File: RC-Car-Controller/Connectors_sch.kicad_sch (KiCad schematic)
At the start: 6 parts, among them J1 MCU_IF, J3 MOTOR_IF, J4 BATT_1, J5 MISC_IF, J6 ANT_IF, J7 BATT2

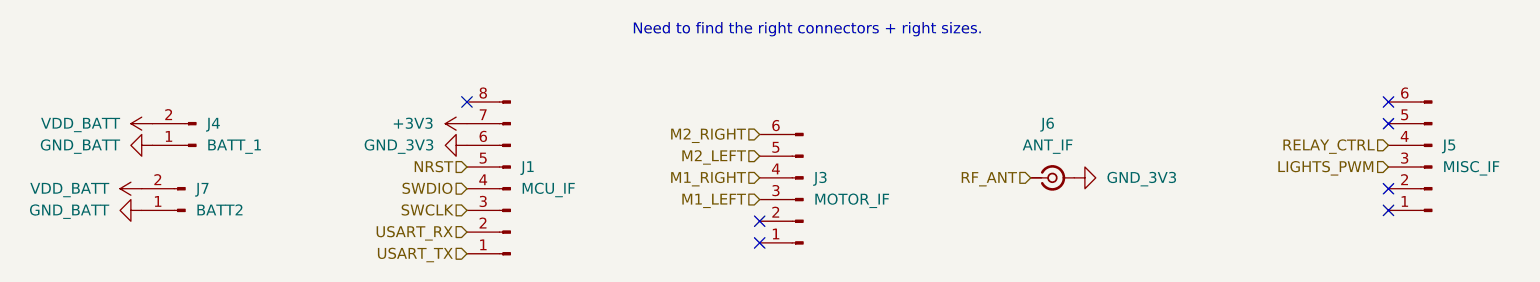
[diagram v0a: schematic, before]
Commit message: Fixed Controller PCB
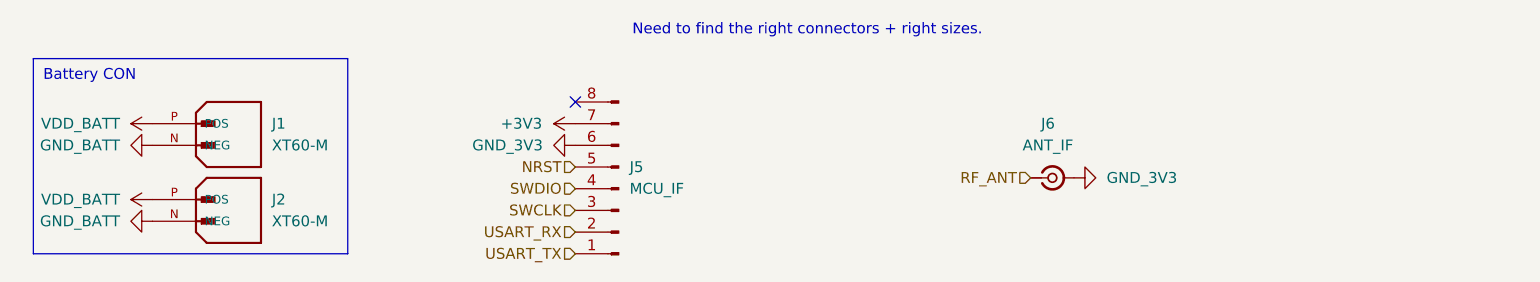
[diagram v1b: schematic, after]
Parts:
- removed J3: MOTOR_IF, symbol Connector:Conn_01x06_Pin
- removed J4: BATT_1, footprints:CONN_1805375_RSP, symbol Connector:Conn_01x02_Pin
- removed J5: MISC_IF, symbol Connector:Conn_01x06_Pin
- removed J7: BATT2, footprints:CONN_1805375_RSP, symbol Connector:Conn_01x02_Pin
- added J1, J2: XT60-M, symbol XT60-M:XT60-M
- renumbered J1 to J5
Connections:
- net GND_BATT: now also J1.N (NEG), J2.N (NEG)
- net VDD_BATT: now also J1.P (POS), J2.P (POS)
- no-connect marks 7 -> 1
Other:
- note added: "Battery CON"
- moved on the sheet: J5

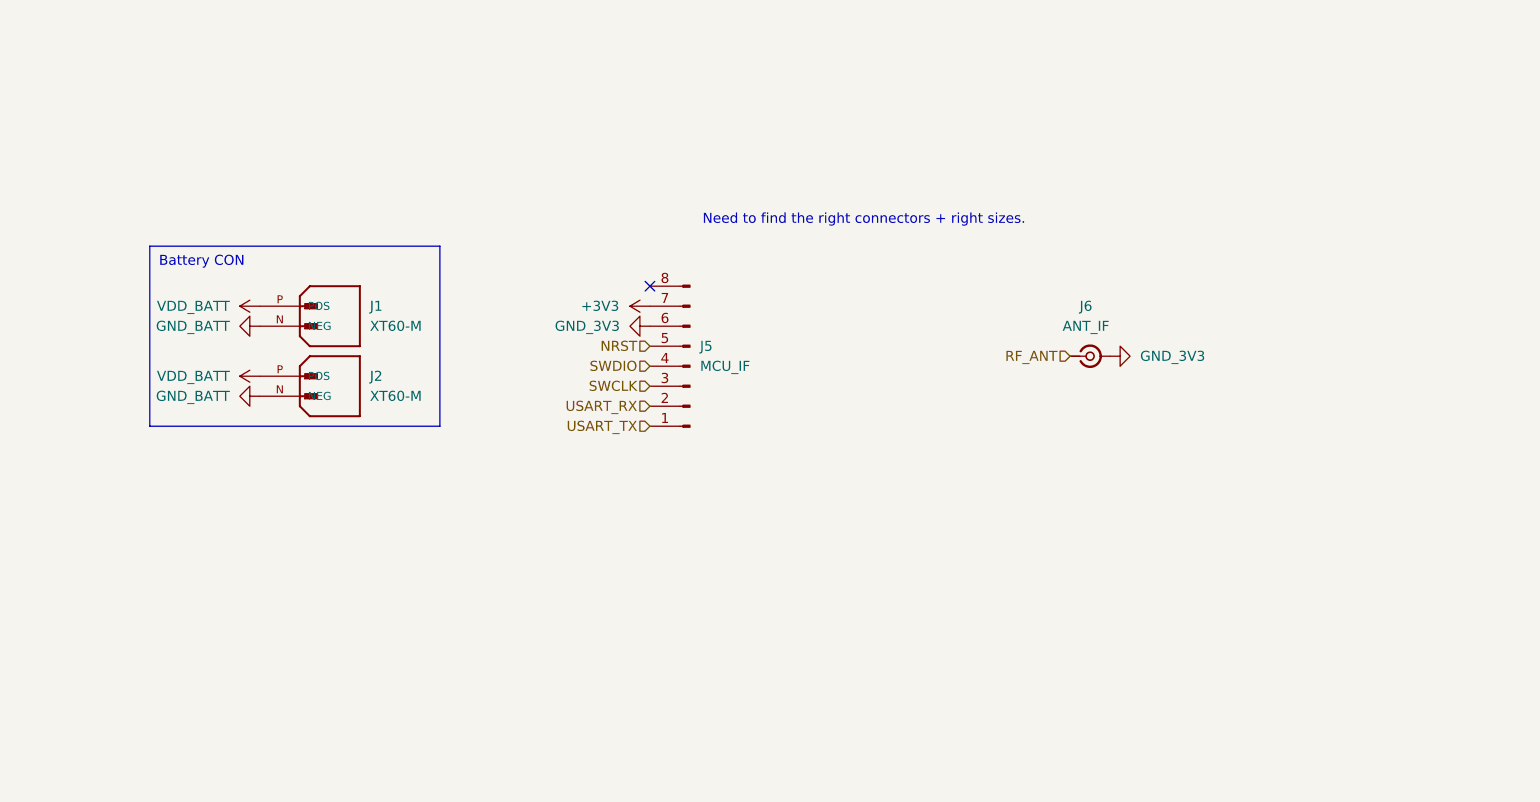
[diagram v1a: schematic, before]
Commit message: Did some stuff on the Controller
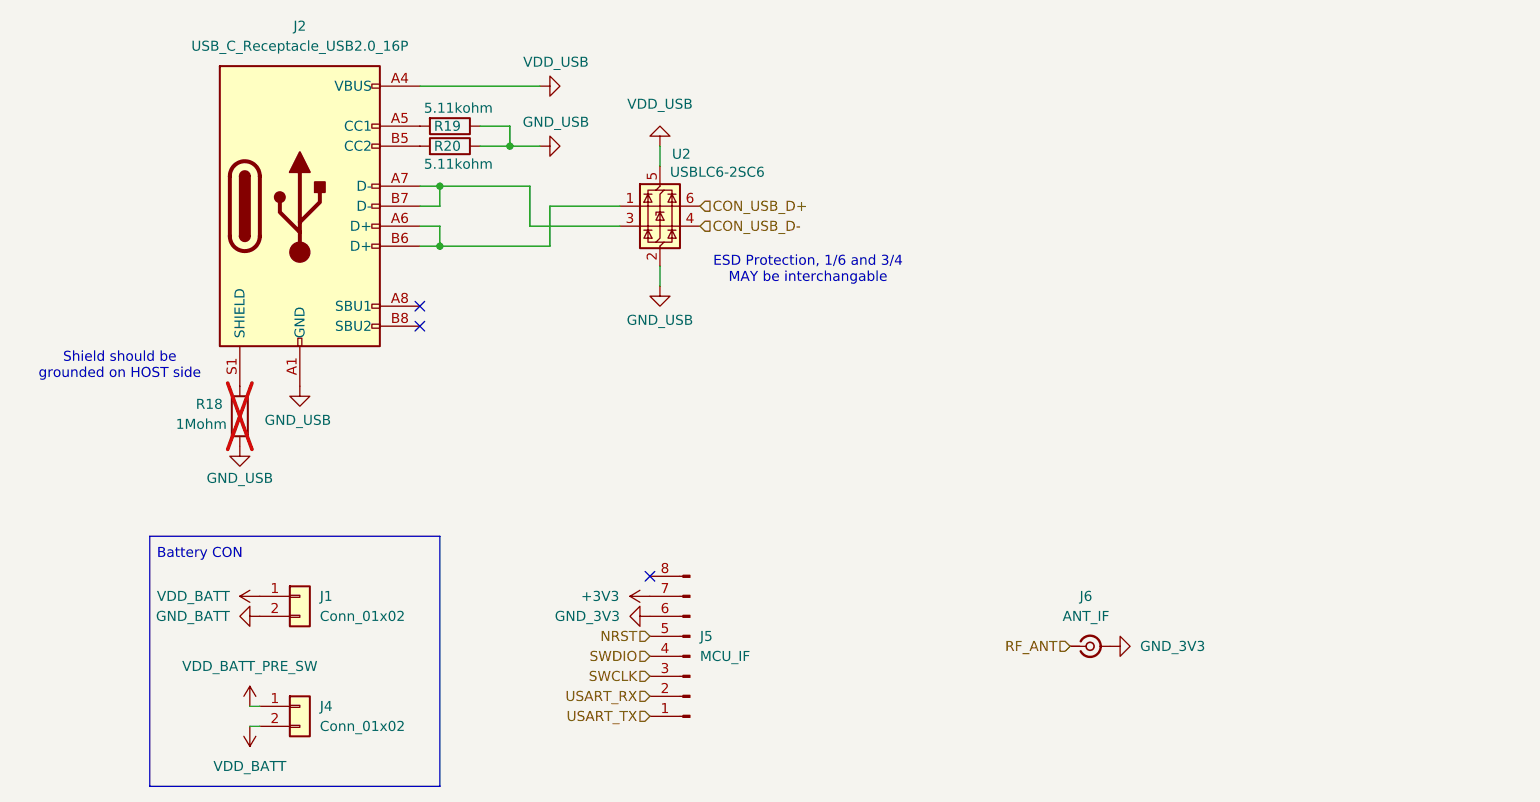
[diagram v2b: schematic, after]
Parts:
- removed J1, J2: XT60-M, symbol XT60-M:XT60-M
- added J1, J4: Conn_01x02, Connector_JST:JST_XH_B2B-XH-AM_1x02_P2.50mm_Vertical, symbol Connector_Generic:Conn_01x02
- added J2: USB_C_Receptacle_USB2.0_16P, symbol Connector:USB_C_Receptacle_USB2.0_16P
- added R18: 1Mohm, Resistor_SMD:R_0603_1608Metric, symbol Device:R
- added R19, R20: 5.11kohm, Resistor_SMD:R_0603_1608Metric, symbol Device:R
- added U2: USBLC6-2SC6, Package_TO_SOT_SMD:SOT-23-6, symbol Power_Protection:USBLC6-2SC6
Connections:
- net GND_BATT: now also J1.2 (Pin_2)
- net VDD_BATT: now also J1.1 (Pin_1), J4.2 (Pin_2)
- new net: J2.A6 (D+), J2.B6 (D+), U2.1 (I/O1)
- new net: J2.A7 (D-), J2.B7 (D-), U2.3 (I/O2)
- new net: J2.A5 (CC1), R19.2
- new net: J2.S1 (SHIELD), R18.1
- new net: J2.B5 (CC2), R20.2
- new net CON_USB_D+: U2.6 (I/O1)
- new net CON_USB_D-: U2.4 (I/O2)
- new net GND_USB: J2.A1 (GND), J2.A12 (GND), J2.B1 (GND), J2.B12 (GND), R18.2, R19.1, R20.1, U2.2 (GND)
- new net VDD_BATT_PRE_SW: J4.1 (Pin_1)
- new net VDD_USB: J2.A4 (VBUS), J2.A9 (VBUS), J2.B4 (VBUS), J2.B9 (VBUS), U2.5 (VBUS)
- no-connect marks 1 -> 3
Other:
- note added: "ESD Protection, 1/6 and 3/4 MAY be interchangable"
- note added: "Shield should be grounded on HOST side"
- note removed: "Need to find the right connectors + right sizes."
- moved on the sheet: J5, J6
